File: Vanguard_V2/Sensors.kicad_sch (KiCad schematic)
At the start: 20 parts, among them IC2 MAX-M10S-00B, IC3 ADXL375BCCZ-RL, IC4 ASM330LHHTR, J7 Conn_Coaxial, U4 LPS22HH, U5 LSM303C

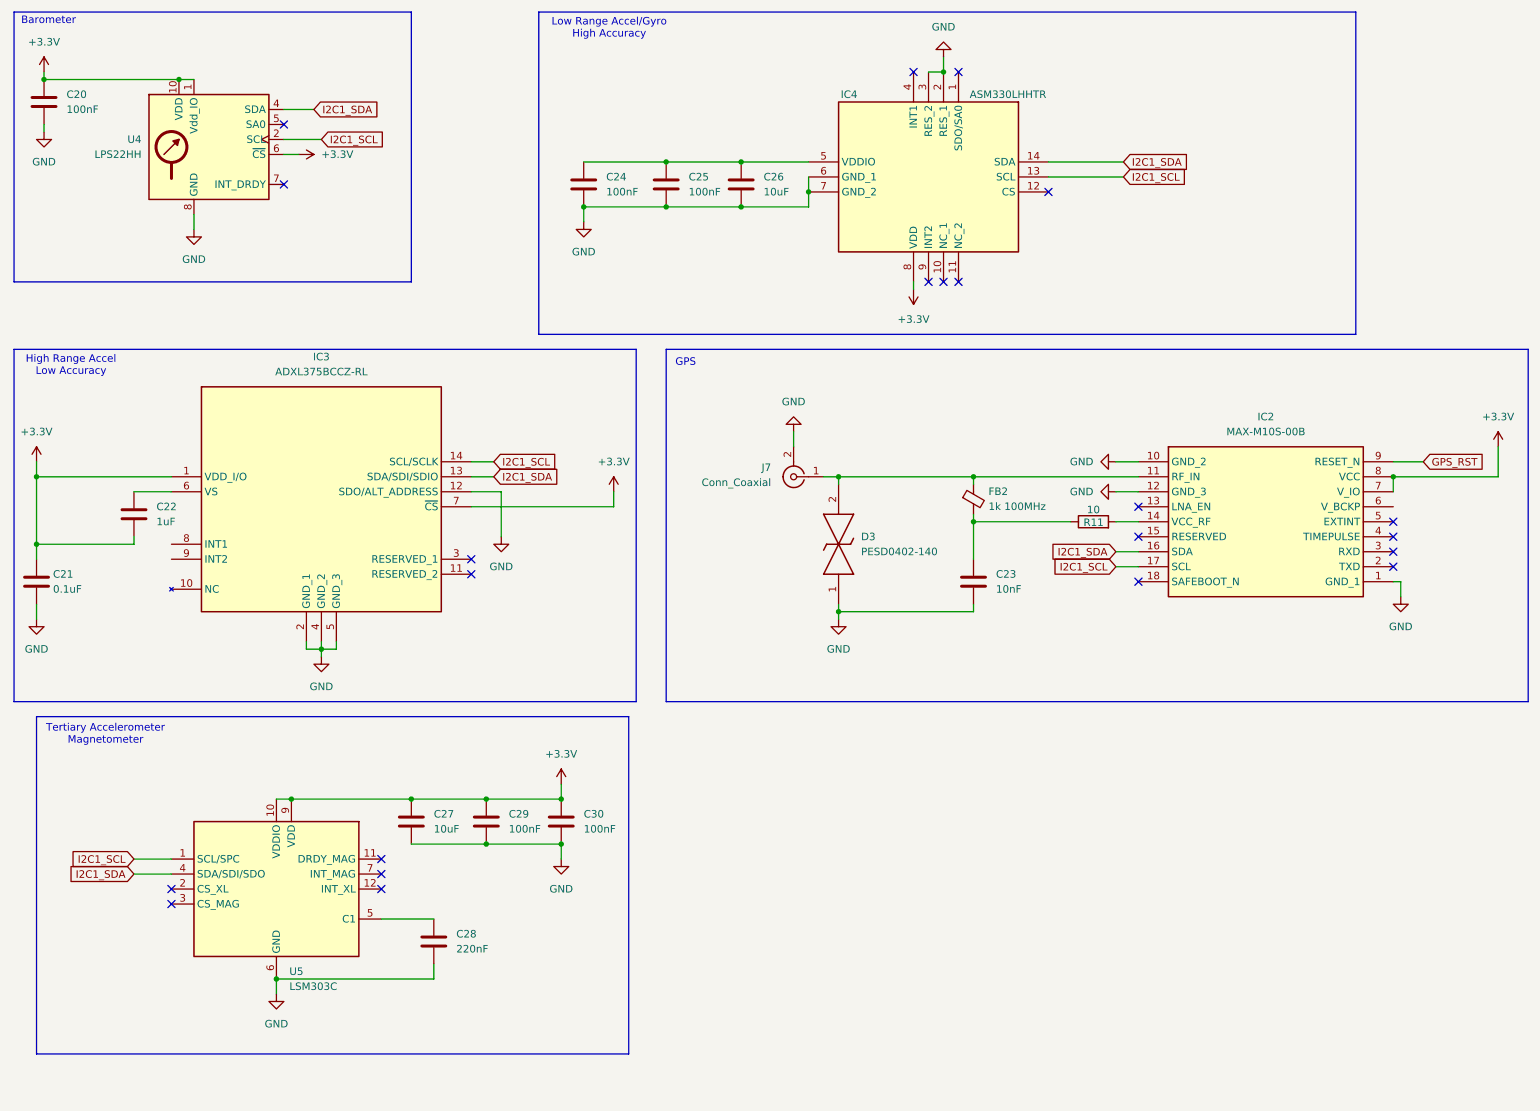
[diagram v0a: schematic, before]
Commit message: V2 Board Ready
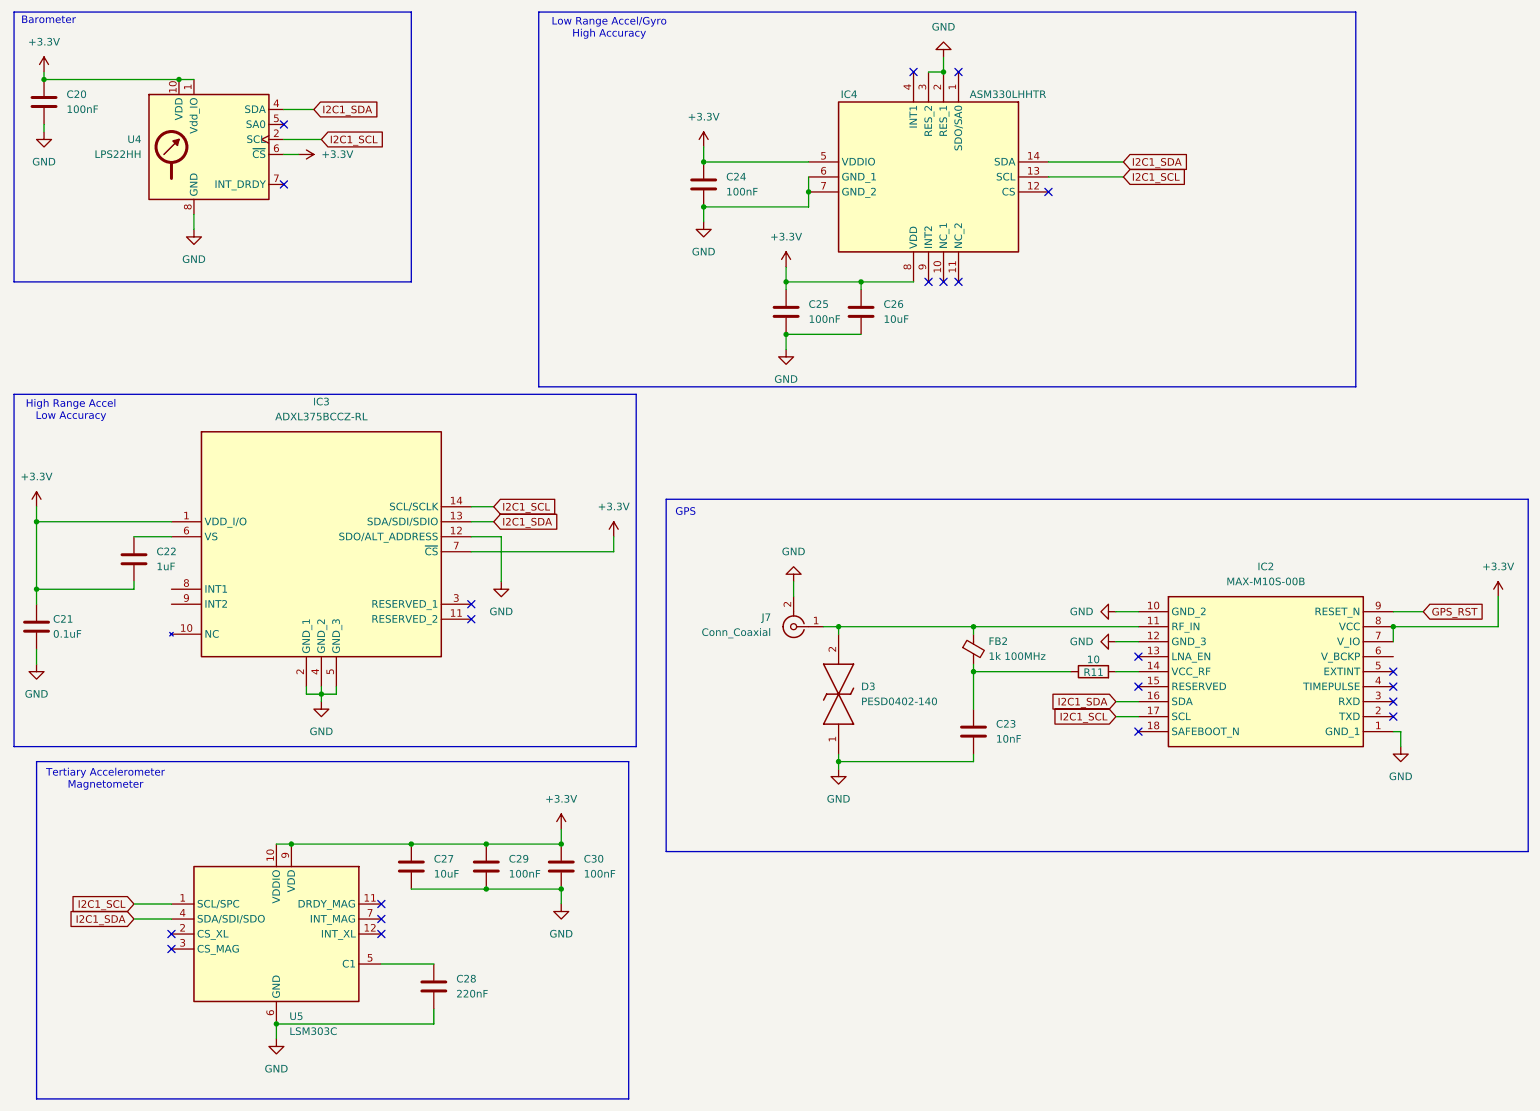
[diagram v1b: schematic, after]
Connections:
- net +3.3V: now also C24.1, C25.1, C26.1, IC4.5 (VDDIO)
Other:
- moved on the sheet: C21, C22, C23, C24, C27, C28, C29, C30, D3, FB2, IC2, IC3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

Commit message: started layout for V2.1
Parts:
- R11: footprint Capacitor_SMD:C_0402_1005Metric -> Resistor_SMD:R_0402_1005Metric
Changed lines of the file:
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@@
 			)
 		)
-		(property "Footprint" "Capacitor_SMD:C_0402_1005Metric"
+		(property "Footprint" "Resistor_SMD:R_0402_1005Metric"
 			(at 196.85 126.238 90)
 			(effects
